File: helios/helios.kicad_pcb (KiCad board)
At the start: 2 copper layers, 150 x 124.5 mm, 67 parts, among them J1 Conn_01x03, J2 Conn_01x04, Q1 BC557, Q2 BC557, Q3 BC557, Q4 BC557, Q5 BC557, Q6 BC557, Q7 BC557, Q8 BC557, SW1 RotaryEncoder_Switch, SW2 SW_Push, SW3 SW_Push, SW4 SW_Push, U1 74HC595, U2 74HC138, U3 CC56-12EWA, U4 74HC595, U5 74HC138, U6 CC56-12EWA

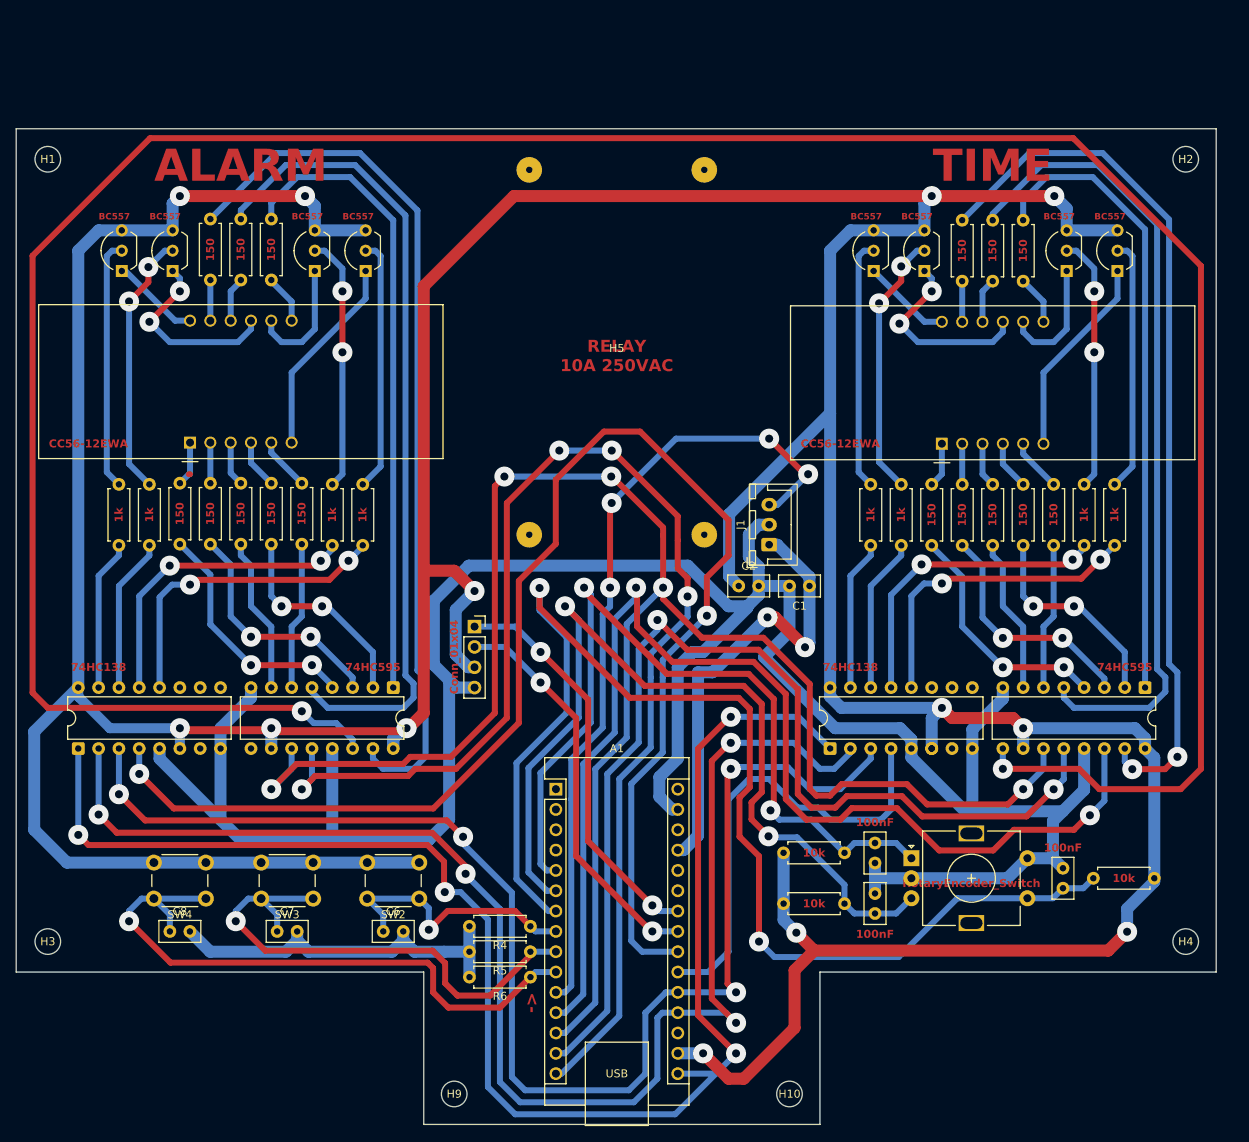
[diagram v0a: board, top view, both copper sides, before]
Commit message: small PCB fixes + print
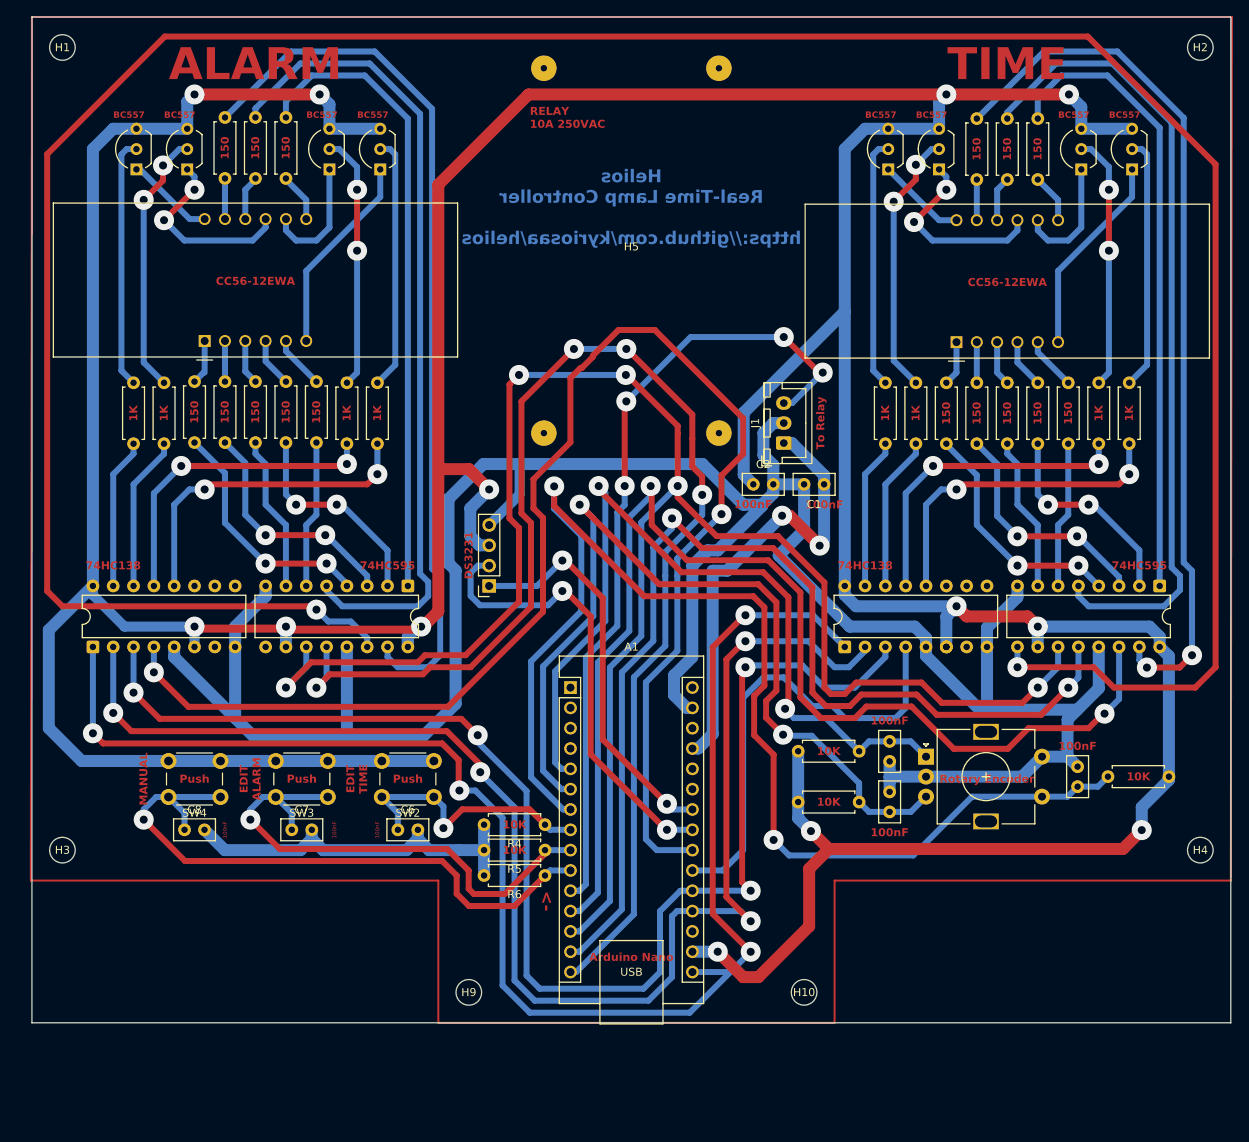
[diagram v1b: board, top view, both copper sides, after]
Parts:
- J1: value Conn_01x03 -> To Relay
- J2: value Conn_01x04 -> DS3231
- R1, R2, R3, R4, R5, R6: value 10k -> 10K
- R10, R27, R28, R29, R30, R7, R8, R9: value 1k -> 1K
- SW1: value RotaryEncoder_Switch -> Rotary Encoder
- moved H1 14.1 mm to (75.5, 36.8)
- moved H2 14.1 mm to (217.7, 36.8)
- moved R5 12.8 mm to (135.8, 137.2)
- moved H5 12.8 mm to (146.6, 62.2)
- moved R1 12.8 mm to (167.5, 124.8)
- moved R10 12.8 mm to (208.8, 78.7)
- moved R17 12.8 mm to (201.2, 86.4)
- moved R19 12.8 mm to (95.8, 45.6)
- moved R20 12.8 mm to (103.4, 45.6)
- moved R21 12.8 mm to (103.4, 86.2)
- moved R22 12.8 mm to (95.8, 86.2)
- moved R23 12.8 mm to (92.0, 86.2)
- moved R24 12.8 mm to (99.6, 45.6)
- moved R25 12.8 mm to (107.2, 86.2)
- moved R26 12.8 mm to (99.6, 86.2)
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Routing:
- net SDA: track 50.2 -> 57.0 mm
- net GND: track 361.0 -> 364.2 mm
- net /Display_Time/DIG4: track 38.5 -> 40.8 mm
- net +3V3: track 651.9 -> 649.6 mm
- net /Display_Time/DIG3: track 37.1 -> 39.3 mm
- net /Display_Alarm/DIG8: track 39.5 -> 40.8 mm
- net ENABLE_ALARM: track 182.2 -> 183.3 mm
- net LATCH_ALARM: track 166.8 -> 167.8 mm
- net SPI_CLK: track 233.7 -> 234.7 mm
- net /Display_Alarm/DIG7: track 38.5 -> 39.3 mm
- net SCL: track 50.5 -> 50.0 mm
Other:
- board size 150 x 124.5 mm -> 149.9 x 125.7 mm
- board text added: "Arduino Nano"
- board text added: "EDIT ALARM"
- board text added: "EDIT TIME"
- board text added: "Helios Real-Time Lamp Controller https://github.com/kyriosaa/helios"
- board text added: "MANUAL"
- board text added: "Push"
